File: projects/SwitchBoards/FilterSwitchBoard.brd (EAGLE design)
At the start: 18.7 x 14.8 mm, 9 parts

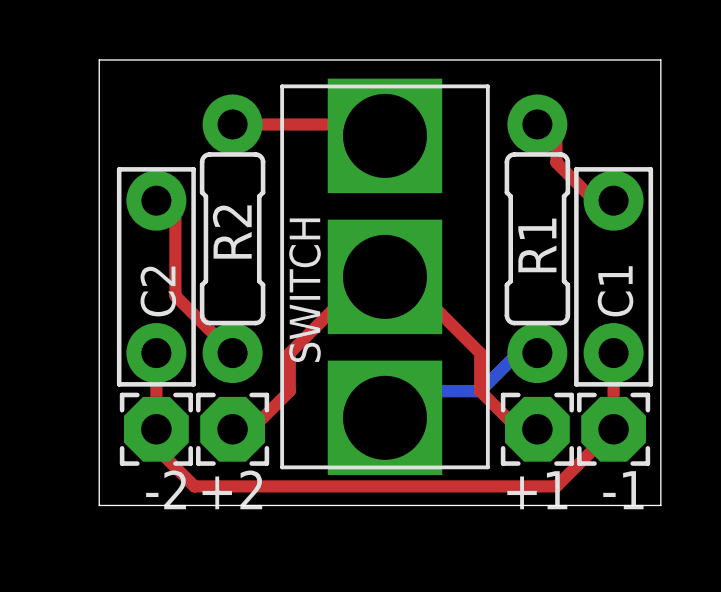
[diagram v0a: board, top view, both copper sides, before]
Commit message: Final project updates. Ready to send to oshpark.
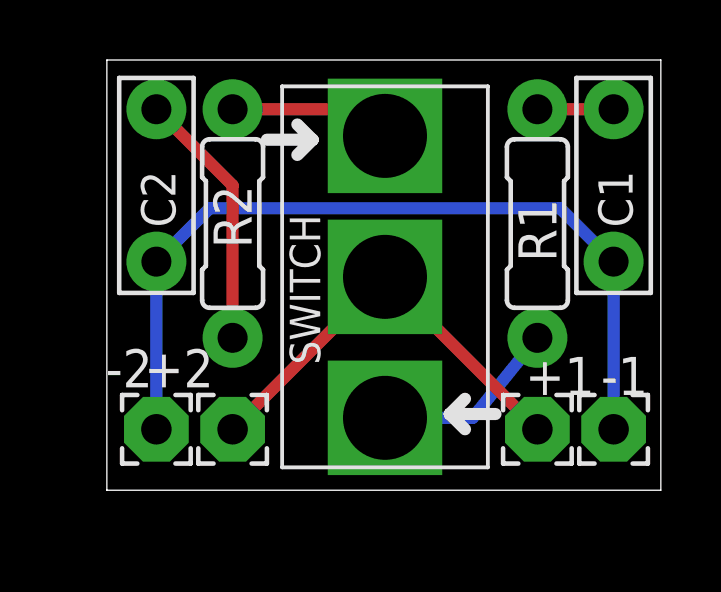
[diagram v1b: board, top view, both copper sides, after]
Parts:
- moved C1 3.05 mm to (17.1, 75.4)
- moved C2 3.05 mm to (1.91, 75.4)
- moved R1 0.51 mm to (14.6, 74.2)
- moved R2 0.51 mm to (4.45, 74.2)
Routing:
- net N$5: track 22.3 -> 27.9 mm
- net N$3: track 6.50 -> 8.67 mm
- net N$2: track 4.34 -> 2.54 mm
- net N$7: track 15.9 -> 14.4 mm
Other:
- board size 18.7 x 14.8 mm -> 18.5 x 14.3 mm
- board text added: "GJCAMANN(C)2014"
- board text added: "V1.0"
- board text removed: "GJCAMANN2014"
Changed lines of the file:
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@@
 <setting verticaltext="up"/>
 </settings>
-<grid distance="0.1" unitdist="inch" unit="inch" style="lines" multiple="1" display="yes" altdistance="0.005" altunitdist="inch" altunit="inch"/>
+<grid distance="0.1" unitdist="inch" unit="inch" style="lines" multiple="1" display="yes" altdistance="0.01" altunitdist="inch" altunit="inch"/>
 <layers>
 <layer number="1" name="Top" color="4" fill="1" visible="yes" active="yes"/>
@@
 <layer number="20" name="Dimension" color="15" fill="1" visible="yes" active="yes"/>
 <layer number="21" name="tPlace" color="7" fill="1" visible="yes" active="yes"/>
-<layer number="22" name="bPlace" color="7" fill="1" visible="yes" active="yes"/>
+<layer number="22" name="bPlace" color="7" fill="1" visible="no" active="yes"/>
 <layer number="23" name="tOrigins" color="15" fill="1" visible="yes" active="yes"/>
 <layer number="24" name="bOrigins" color="15" fill="1" visible="yes" active="yes"/>
@@
 <board>
 <plain>
-<wire x1="0" y1="64.77" x2="18.72" y2="64.77" width="0" layer="20"/>
-<wire x1="18.72" y1="64.77" x2="18.72" y2="79.619" width="0" layer="20"/>
-<wire x1="18.72" y1="79.619" x2="0" y2="79.619" width="0" layer="20"/>
-<wire x1="0" y1="79.619" x2="0" y2="64.77" width="0" layer="20"/>
+<wire x1="0.254" y1="65.278" x2="18.72" y2="65.278" width="0" layer="20"/>
+<wire x1="18.72" y1="65.278" x2="18.72" y2="79.619" width="0" layer="20"/>
+<wire x1="18.72" y1="79.619" x2="0.254" y2="79.619" width="0" layer="20"/>
+<wire x1="0.254" y1="79.619" x2="0.254" y2="65.278" width="0" layer="20"/>
 <text x="7.62" y="78.105" size="1.016" layer="22" rot="MR270">FilterSwitchBoard</text>
-<text x="11.43" y="66.04" size="1.016" layer="22" rot="MR90">GJCAMANN2014</text>
+<text x="11.43" y="66.04" size="1.016" layer="22" rot="MR90">GJCAMANN(C)2014</text>
+<text x="18.669" y="70.104" size="1.016" layer="22" rot="MR0">V1.0</text>
+<wire x1="5.588" y1="76.962" x2="7.112" y2="76.962" width="0.4064" layer="21"/>
+<wire x1="6.604" y1="77.47" x2="7.112" y2="76.962" width="0.4064" layer="21"/>
+<wire x1="7.112" y1="76.962" x2="6.604" y2="76.454" width="0.4064" layer="21"/>
+<wire x1="13.208" y1="67.818" x2="11.684" y2="67.818" width="0.4064" layer="21"/>
+<wire x1="12.192" y1="68.326" x2="11.684" y2="67.818" width="0.4064" layer="21"/>
+<wire x1="11.684" y1="67.818" x2="12.192" y2="67.31" width="0.4064" layer="21"/>
 </plain>
 <attributes>
@@
 <elements>
 <element name="U$1" library="gc_pedal_parts" package="SPDT_SOLDER" value="SPDT_SOLDER" x="9.525" y="72.39"/>
-<element name="R1" library="resistors" package="R0207/3" value="" x="14.605" y="73.66" rot="R90"/>
-<element name="R2" library="resistors" package="R0207/3" value="" x="4.445" y="73.66" rot="R270"/>
-<element name="C1" library="capacitors-film" package="BOX_SMALL" value="" x="17.145" y="72.39" rot="R90"/>
-<element name="C2" library="capacitors-film" package="BOX_SMALL" value="" x="1.905" y="72.39" rot="R90"/>
-<element name="+2" library="wirepad" package="2,15/1,0" value="" x="4.445" y="67.31" rot="R180"/>
-<element name="-1" library="wirepad" package="2,15/1,0" value="" x="17.145" y="67.31" rot="R180"/>
-<element name="-2" library="wirepad" package="2,15/1,0" value="" x="1.905" y="67.31" rot="R180"/>
-<element name="+1" library="wirepad" package="2,15/1,0" value="" x="14.605" y="67.31" rot="R180"/>
+<element name="R1" library="resistors" package="R0207/3" value="" x="14.605" y="74.168" rot="R90"/>
+<element name="R2" library="resistors" package="R0207/3" value="" x="4.445" y="74.168" rot="R270"/>
+<element name="C1" library="capacitors-film" package="BOX_SMALL" value="" x="17.145" y="75.438" rot="R90"/>
+<element name="C2" library="capacitors-film" package="BOX_SMALL" value="" x="1.905" y="75.438" rot="R90"/>
+<element name="+2" library="wirepad" package="2,15/1,0" value="" x="4.445" y="67.31" smashed="yes" rot="R180">
+<attribute name="NAME" x="3.81" y="69.977" size="1.27" layer="25" ratio="10" rot="R180"/>
+<attribute name="VALUE" x="4.445" y="66.31" size="0.0254" layer="27" rot="R180"/>
+</element>
+<element name="-1" library="wirepad" package="2,15/1,0" value="" x="17.145" y="67.31" smashed="yes" rot="R180">
+<attribute name="NAME" x="18.288" y="69.723" size="1.27" layer="25" ratio="10" rot="R180"/>
+<attribute name="VALUE" x="17.145" y="66.31" size="0.0254" layer="27" rot="R180"/>
+</element>
+<element name="-2" library="wirepad" package="2,15/1,0" value="" x="1.905" y="67.31" smashed="yes" rot="R180">
+<attribute name="NAME" x="1.778" y="69.977" size="1.27" layer="25" ratio="10" rot="R180"/>
+<attribute name="VALUE" x="1.905" y="66.31" size="0.0254" layer="27" rot="R180"/>
+</element>
+<element name="+1" library="wirepad" package="2,15/1,0" value="" x="14.605" y="67.31" smashed="yes" rot="R180">
+<attribute name="NAME" x="16.51" y="69.723" size="1.27" layer="25" ratio="10" rot="R180"/>
+<attribute name="VALUE" x="14.605" y="66.31" size="0.0254" layer="27" rot="R180"/>
+</element>
 </elements>
 <signals>
@@
 <contactref element="U$1" pad="P$1"/>
 <contactref element="R1" pad="1"/>
-<wire x1="12.7" y1="68.58" x2="13.97" y2="69.85" width="0.4064" layer="16"/>
-<wire x1="10.16" y1="68.58" x2="12.7" y2="68.58" width="0.4064" layer="16"/>
-<wire x1="13.97" y1="69.85" x2="14.605" y2="69.85" width="0.1524" layer="16"/>
-<wire x1="10.16" y1="68.58" x2="9.525" y2="67.691" width="0.1524" layer="16"/>
+<wire x1="9.525" y1="67.691" x2="12.446" y2="67.691" width="0.4064" layer="16"/>
+<wire x1="12.446" y1="67.691" x2="14.605" y2="70.358" width="0.4064" layer="16"/>
 </signal>
 <signal name="N$2">
 <contactref element="R1" pad="2"/>
 <contactref element="C1" pad="2"/>
-<wire x1="15.24" y1="76.2" x2="16.51" y2="74.93" width="0.4064" layer="1"/>
-<wire x1="15.24" y1="77.47" x2="15.24" y2="76.2" width="0.4064" layer="1"/>
-<wire x1="16.51" y1="74.93" x2="17.145" y2="74.93" width="0.4064" layer="1"/>
-<wire x1="15.24" y1="77.47" x2="14.605" y2="77.47" width="0.1524" layer="1"/>
+<wire x1="14.605" y1="77.978" x2="17.145" y2="77.978" width="0.4064" layer="1"/>
 </signal>
 <signal name="N$3">
 <contactref element="R2" pad="2"/>
 <contactref element="C2" pad="2"/>
-<wire x1="2.54" y1="71.755" x2="3.81" y2="70.485" width="0.4064" layer="1"/>
-<wire x1="2.54" y1="74.93" x2="2.54" y2="71.755" width="0.4064" layer="1"/>
-<wire x1="3.81" y1="70.485" x2="4.445" y2="69.85" width="0.1524" layer="1"/>
-<wire x1="2.54" y1="74.93" x2="1.905" y2="74.93" width="0.1524" layer="1"/>
+<wire x1="1.905" y1="77.978" x2="4.445" y2="75.438" width="0.4064" layer="1"/>
+<wire x1="4.445" y1="75.438" x2="4.445" y2="70.358" width="0.4064" layer="1"/>
 </signal>
 <signal name="N$4">
 <contactref element="U$1" pad="P$2"/>
 <contactref element="R2" pad="1"/>
-<wire x1="8.89" y1="77.47" x2="4.445" y2="77.47" width="0.4064" layer="1"/>
-<wire x1="8.89" y1="77.47" x2="9.525" y2="77.089" width="0.4064" layer="1"/>
+<wire x1="4.445" y1="77.978" x2="8.636" y2="77.978" width="0.4064" layer="1"/>
+<wire x1="8.636" y1="77.978" x2="9.525" y2="77.089" width="0.4064" layer="1"/>
 </signal>
 <signal name="N$5">
@@
 <contactref element="-1" pad="1"/>
 <contactref element="-2" pad="1"/>
-<wire x1="1.905" y1="67.31" x2="1.905" y2="66.675" width="0.4064" layer="1"/>
-<wire x1="1.905" y1="66.675" x2="3.175" y2="65.405" width="0.4064" layer="1"/>
-<wire x1="3.175" y1="65.405" x2="15.24" y2="65.405" width="0.4064" layer="1"/>
-<wire x1="15.24" y1="65.405" x2="17.145" y2="67.31" width="0.4064" layer="1"/>
-<wire x1="1.905" y1="69.85" x2="1.905" y2="67.31" width="0.4064" layer="1"/>
-<wire x1="17.145" y1="69.85" x2="17.145" y2="67.31" width="0.4064" layer="1"/>
+<wire x1="1.905" y1="67.31" x2="1.905" y2="72.898" width="0.4064" layer="16"/>
+<wire x1="17.145" y1="72.898" x2="17.145" y2="67.31" width="0.4064" layer="16"/>
+<wire x1="1.905" y1="72.898" x2="3.683" y2="74.676" width="0.4064" layer="16"/>
+<wire x1="3.683" y1="74.676" x2="15.367" y2="74.676" width="0.4064" layer="16"/>
+<wire x1="15.367" y1="74.676" x2="17.145" y2="72.898" width="0.4064" layer="16"/>
 </signal>
 <signal name="N$7">
@@
 <contactref element="+2" pad="1"/>
 <contactref element="+1" pad="1"/>
-<wire x1="6.35" y1="68.58" x2="5.08" y2="67.31" width="0.4064" layer="1"/>
-<wire x1="6.35" y1="69.85" x2="6.35" y2="68.58" width="0.4064" layer="1"/>
-<wire x1="8.89" y1="72.39" x2="6.35" y2="69.85" width="0.4064" layer="1"/>
-<wire x1="5.08" y1="67.31" x2="4.445" y2="67.31" width="0.1524" layer="1"/>
-<wire x1="8.89" y1="72.39" x2="9.525" y2="72.39" width="0.4064" layer="1"/>
-<wire x1="12.7" y1="68.58" x2="13.97" y2="67.31" width="0.4064" layer="1"/>
-<wire x1="12.7" y1="69.85" x2="12.7" y2="68.58" width="0.4064" layer="1"/>
-<wire x1="10.16" y1="72.39" x2="12.7" y2="69.85" width="0.4064" layer="1"/>
-<wire x1="13.97" y1="67.31" x2="14.605" y2="67.31" width="0.4064" layer="1"/>
-<wire x1="10.16" y1="72.39" x2="9.525" y2="72.39" width="0.1524" layer="1"/>
+<wire x1="4.445" y1="67.31" x2="9.525" y2="72.39" width="0.4064" layer="1"/>
+<wire x1="9.525" y1="72.39" x2="14.605" y2="67.31" width="0.4064" layer="1"/>
 </signal>
 </signals>
